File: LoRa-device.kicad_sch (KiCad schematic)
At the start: 121 parts, among them J1 Connector, USB-TYPE-C-16P, J2 Conn_01x02_Pin, J3 Conn_Coaxial, J4 Conn_01x14_Pin, J6 Conn_01x04_Pin, J7 Screw_Terminal_01x08, J8 U.FL, Q2 S8050, SW2 SW_DPST_x2, U1 ESP32-S3, U10 TPS2116DRL, U11 L76KB-A58, U13 MCP23S17_ML, U2 W25Q128JVS, U3 TP4055, U5 Ai-Thinker-Ra-01, U6 USBLC6-2P6, U7 STLQ015M33R, U8 TPS22917LDBV, U9 AP63203WU, Y1 32.768 kHz, Y2 40MHz(10ppm)

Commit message: Major overhaul of version A
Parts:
- removed C30: 1uF, PCM_JLCPCB:C_0402, symbol PCM_JLCPCB-Capacitors:0402,1uF
- removed J1: Connector, USB-TYPE-C-16P, PCM_JLCPCB:TYPE-C-SMD_HX-TYPE-C-16PIN, symbol PCM_JLCPCB-Extended:Connector, USB-TYPE-C-16P
- removed J7: Screw_Terminal_01x08, Connector_Phoenix_MC:PhoenixContact_MC_1,5_8-G-3.81_1x08_P3.81mm_Horizontal, symbol Connector:Screw_Terminal_01x08
- removed R14, R17: 5.1K, Resistor_SMD:R_0402_1005Metric, symbol Device:R
- removed R40: 100kΩ, PCM_JLCPCB:R_0402, symbol PCM_JLCPCB-Resistors:0402,100kΩ
- removed R41: 47Ω, PCM_JLCPCB:R_0402, symbol PCM_JLCPCB-Resistors:0402,47Ω
- removed TP2: TestPoint_2Pole, TestPoint:TestPoint_2Pads_Pitch2.54mm_Drill0.8mm, symbol Connector:TestPoint_2Pole
- added J1: Micro_SD_Card_Det1, Lora-device:TF-SMD_TF-01A, symbol Connector:Micro_SD_Card_Det1
- added MK1: SPH0645LM4H, Sensor_Audio:Knowles_SPH0645LM4H-6_3.5x2.65mm, symbol Sensor_Audio:SPH0645LM4H
- added R34, R35: 5.1K, Resistor_SMD:R_0402_1005Metric, symbol Device:R
- added U4: MC-121-L119, Lora-device:USB-C-SMD_HANBO_MC-121-L119, symbol Lora-device:MC-121-L119
- J3: footprint Connector_Coaxial:SMA_Molex_73251-1153_EdgeMount_Horizontal -> Lora-device:SMA-SMD_BWSMA-KE-P001
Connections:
- net +5V: now also U4.A4B9 (VBUS), U4.B4A9 (VBUS)
- net GND: now also R34.1, R35.1, U4.13 (EH), U4.A1B12 (GND), U4.B1A12 (GND)
- net MOSIA: no longer J6.2 (Pin_2)
- net SCKA: no longer J6.4 (Pin_4)
- net SCREEN_CS: now also U13.1 (GPB4); no longer U1.15 (GPIO10)
- net SD_CS: now also U13.24 (GPA7); no longer J6.1 (Pin_1), U1.12 (GPIO7)
- net TOUCH_CS: now also U13.2 (GPB5); no longer U1.24 (GPIO18)
- net LORA_IO4: now reaches U5.10 (DIO4)
- net LORA_IO4: now also U13.27 (GPB2)
- net LORA_IO5: now reaches U5.11 (DIO5)
- net LORA_IO5: now also U13.28 (GPB3)
- net GPS_1PPS: now reaches U11.4 (1PPS)
- net GPS_1PPS: now also U1.12 (GPIO7)
- net LORA_IO2: now reaches U5.7 (DIO2)
- net LORA_IO2: now also U13.25 (GPB0)
- net LORA_IO3: now reaches U5.8 (DIO3)
- net LORA_IO3: now also U13.26 (GPB1)
- net at U6.1 (I/O1): now also U4.A7 (DN1), U4.B7 (DN2)
- net at U6.3 (I/O2): now also U4.A6 (DP1), U4.B6 (DP2)
- net IO18: now reaches U13.15 (INTB)
- net IO18: now also U1.24 (GPIO18)
- net IO10: now reaches U13.16 (INTA)
- net IO10: now also U1.15 (GPIO10)
- net GPB6: now reaches U13.3 (GPB6)
- net GPB7: now reaches U13.4 (GPB7)
- new net: R34.2, U4.A5 (CC1)
- new net: R35.2, U4.B5 (CC2)
- no-connect marks 22 -> 17
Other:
- note added: "HEADER"
- note added: "I2S MICROPHONE"
- note added: "ILI9341"
- note added: "MICRO SD CARD"
- note removed: "HEADER PINS"
- note removed: "ILI9341/SD CARD"
- moved on the sheet: BZ1, C13, C16, C17, C3, C32, C36, C39, C40, C6, C7, D2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

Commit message: Just a backup.
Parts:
- removed MK1: SPH0645LM4H, Sensor_Audio:Knowles_SPH0645LM4H-6_3.5x2.65mm, symbol Sensor_Audio:SPH0645LM4H
- added C30: 100nF, PCM_JLCPCB:C_0402, symbol PCM_JLCPCB-Capacitors:0402,100nF
- added C44: 220pF, PCM_JLCPCB:C_0402, symbol PCM_JLCPCB-Capacitors:0402,220pF
- added C45: 1uF, PCM_JLCPCB:C_0402, symbol PCM_JLCPCB-Capacitors:0402,1uF
- added J5: Conn_01x07_Pin, Connector_PinSocket_2.54mm:PinSocket_1x07_P2.54mm_Horizontal, symbol Connector:Conn_01x07_Pin
- added R14, R17, R37: 10K, Resistor_SMD:R_0402_1005Metric, symbol Device:R
- added R38, R39, R40: 33Ω, PCM_JLCPCB:R_0805, symbol PCM_JLCPCB-Resistors:0805,33Ω
- added R41, R42: 4.7kΩ, PCM_JLCPCB:R_0402, symbol PCM_JLCPCB-Resistors:0402,4.7kΩ
- added SW1, SW3: CK_KMS2xxGP, Button_Switch_SMD:SW_SPST_CK_KMS2xxGP, symbol Switch:CK_KMS2xxGP
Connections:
- net +3V3: now also J1.4 (VDD), C30.1, C44.1, C45.1, J5.7 (Pin_7), R14.1, R17.1, R37.1, R41.1, R42.1
- net GND: now also J1.10 (SHIELD), J1.6 (VSS), C30.2, C44.2, C45.2, J5.6 (Pin_6), SW1.1, SW1.SH (B), SW3.1, SW3.SH (B)
- net GPB6: now also J1.9 (DET)
- net GPB7: now also SW1.2
- net IO1: now also J5.3 (Pin_3), R40.1; no longer U1.6 (GPIO1)
- net IO17: now also SW3.2
- net IO4: now also J5.4 (Pin_4), R39.1; no longer U1.9 (GPIO4)
- net IO8: now also R38.2
- net MISOA: now also J1.7 (DAT0), R14.2
- net MOSIA: now also J1.3 (CMD)
- net SCKA: now also J1.5 (CLK)
- net SD_CS: now also J1.2 (DAT3/CD)
- net U0RXD/IO44: now also J5.2 (Pin_2), R41.2
- net U0TXD/IO43: now also J5.1 (Pin_1), R42.2
- net at J1.1 (DAT2): now also R17.2
- net at J1.8 (DAT1): now also R37.2
- new net: R40.2, U1.6 (GPIO1)
- new net: R39.2, U1.9 (GPIO4)
- new net: J5.5 (Pin_5), R38.1
- no-connect marks 17 -> 21
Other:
- note added: "BUTTONS"
- note added: "I2S/I2C HEADER"
- note removed: "I2S MICROPHONE"
- moved on the sheet: C33, J1, J6

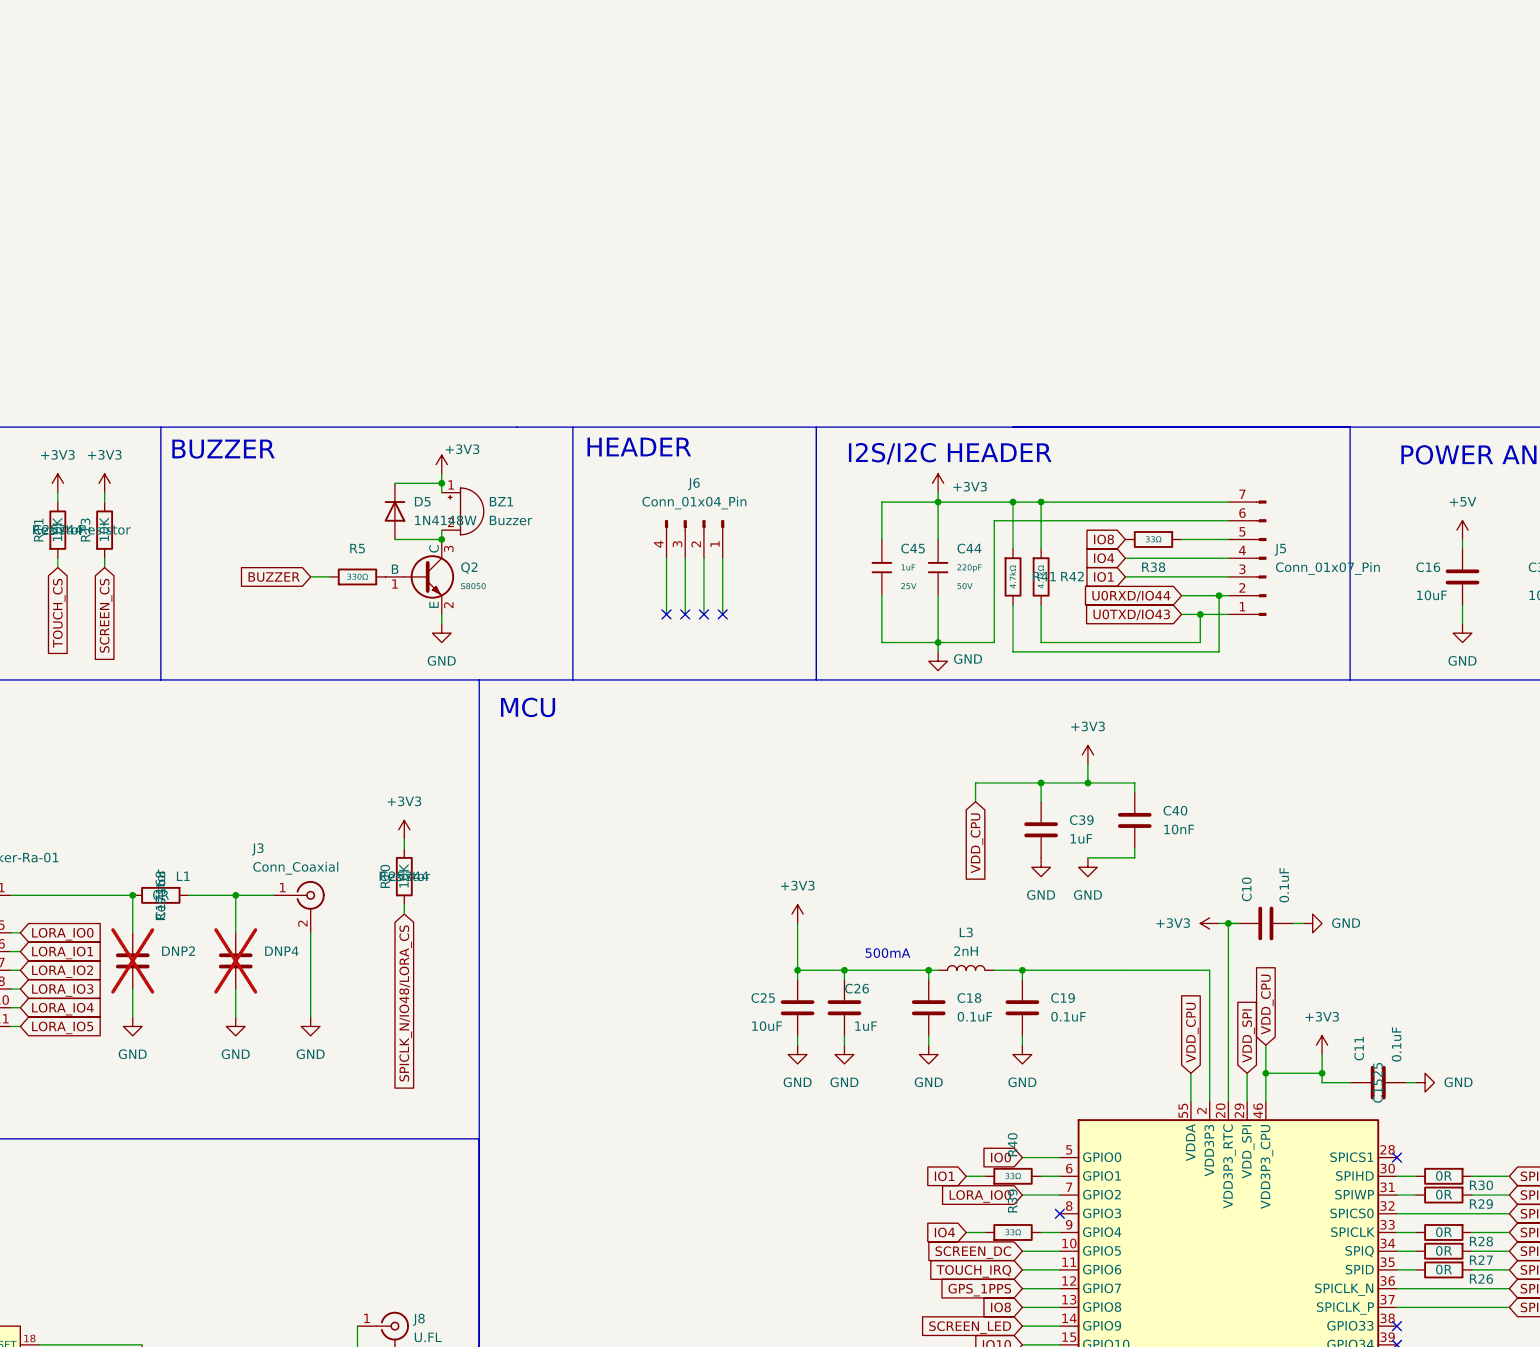
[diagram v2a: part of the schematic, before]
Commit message: Cleanup and update project files.
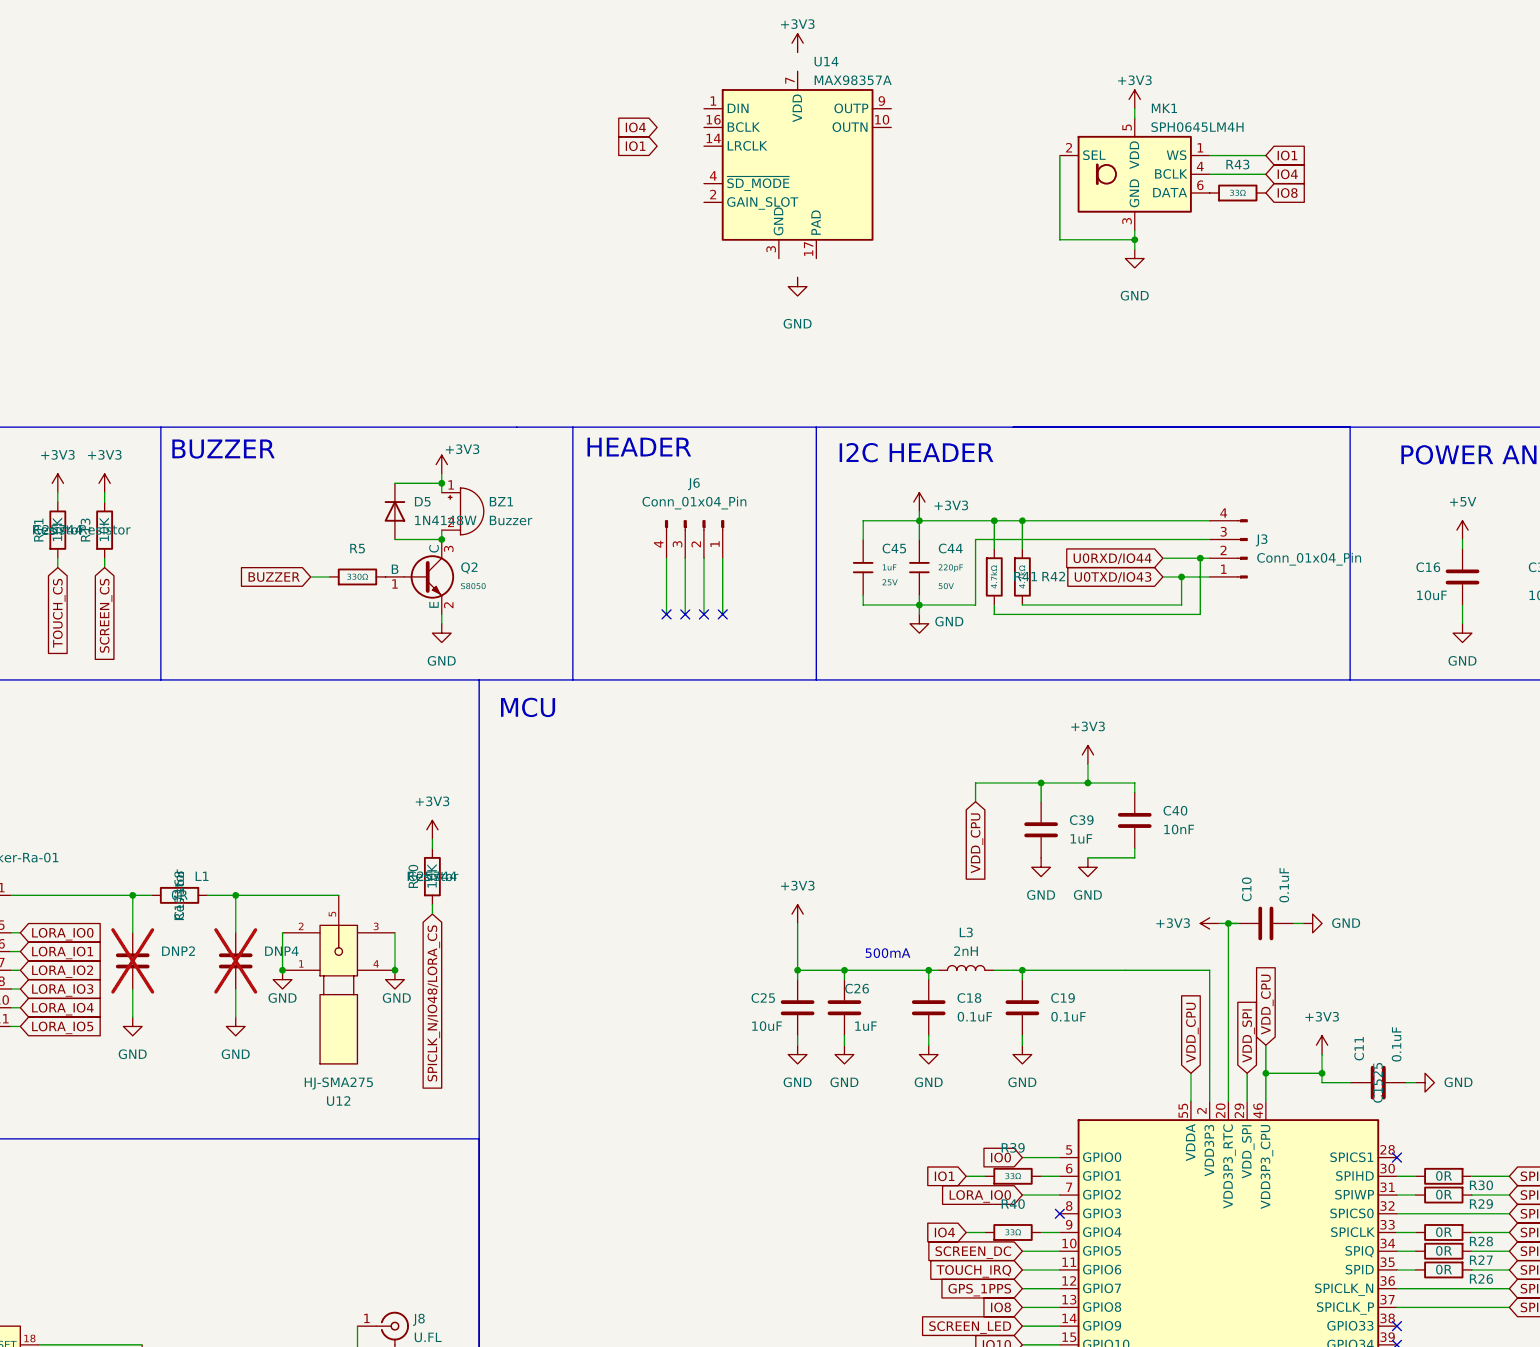
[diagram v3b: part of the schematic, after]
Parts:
- removed J3: Conn_Coaxial, Lora-device:SMA-SMD_BWSMA-KE-P001, symbol Connector:Conn_Coaxial
- removed J5: Conn_01x07_Pin, Connector_PinSocket_2.54mm:PinSocket_1x07_P2.54mm_Horizontal, symbol Connector:Conn_01x07_Pin
- removed R38, R39, R40: 33Ω, PCM_JLCPCB:R_0805, symbol PCM_JLCPCB-Resistors:0805,33Ω
- added J3: Conn_01x04_Pin, Connector_PinSocket_2.54mm:PinSocket_1x04_P2.54mm_Horizontal, symbol Connector:Conn_01x04_Pin
- added MK1: SPH0645LM4H, Sensor_Audio:Knowles_SPH0645LM4H-6_3.5x2.65mm, symbol Sensor_Audio:SPH0645LM4H
- added R39, R40, R43: 33Ω, PCM_JLCPCB:R_0402, symbol PCM_JLCPCB-Resistors:0402,33Ω
- added U12: HJ-SMA275, my_footprints:SMA-SMD_BWSMA-KE-P001, symbol SMA_connector:HJ-SMA275
- added U14: MAX98357A, Package_DFN_QFN:TQFN-16-1EP_3x3mm_P0.5mm_EP1.23x1.23mm, symbol Audio:MAX98357A
- J1: footprint Lora-device:TF-SMD_TF-01A -> my_footprints:TF-SMD_TF-01A
- SW1, SW3: LCSC (none) -> C221698
- U11: footprint Lora-device:GPSM-SMD_18P-L10.1-W9.7-P1.10 -> my_footprints:GPSM-SMD_18P-L10.1-W9.7-P1.10
- U4: footprint Lora-device:USB-C-SMD_HANBO_MC-121-L119 -> my_footprints:USB-C-SMD_HANBO_MC-121-L119
- U7: footprint Lora-device:SOT-23-5_L3.0-W1.7-P0.95-LS2.8-BR -> my_footprints:SOT-23-5_L3.0-W1.7-P0.95-LS2.8-BR
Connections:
- net +3V3: now also J3.4 (Pin_4), MK1.5 (VDD)
- net GND: now also J3.3 (Pin_3), MK1.2 (SEL), MK1.3 (GND), U12.1, U12.2, U12.3, U12.4
- net IO1: now also MK1.1 (WS), R39.1
- net IO4: now also MK1.4 (BCLK), R40.1
- net IO8: now also R43.2
- net U0RXD/IO44: now also J3.2 (Pin_2)
- net U0TXD/IO43: now also J3.1 (Pin_1)
- net at U1.6 (GPIO1): now also R39.2
- net at U1.9 (GPIO4): now also R40.2
- net at DNP4.1, L1.2: now also U12.5
- new net: MK1.6 (DATA), R43.1
- new net: U14.11 (GND), U14.15 (GND), U14.3 (GND)
- new net: U14.7 (VDD), U14.8 (VDD)
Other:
- note added: "I2C HEADER"
- note removed: "I2S/I2C HEADER"
- moved on the sheet: C44, C45, L1, R10, R41, R42
